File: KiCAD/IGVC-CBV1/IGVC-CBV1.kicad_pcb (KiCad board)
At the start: 2 copper layers, 9.8 x 4.5 mm, 42 parts, among them IC1 STM32F407ZGT6, IC2 SPX3819M5-L-3-3_TR, IC3 AT45DB081E-SSHN-B, J1 STLINKV2 PINS (2.54mm Pitch), J2 Motor Driver Pins (2.54mm Pit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, J3 12401948E412A, J4 Conn_01x02, SW1 SW_SPDT, Y1 EB2532YA12-25.000M_TR

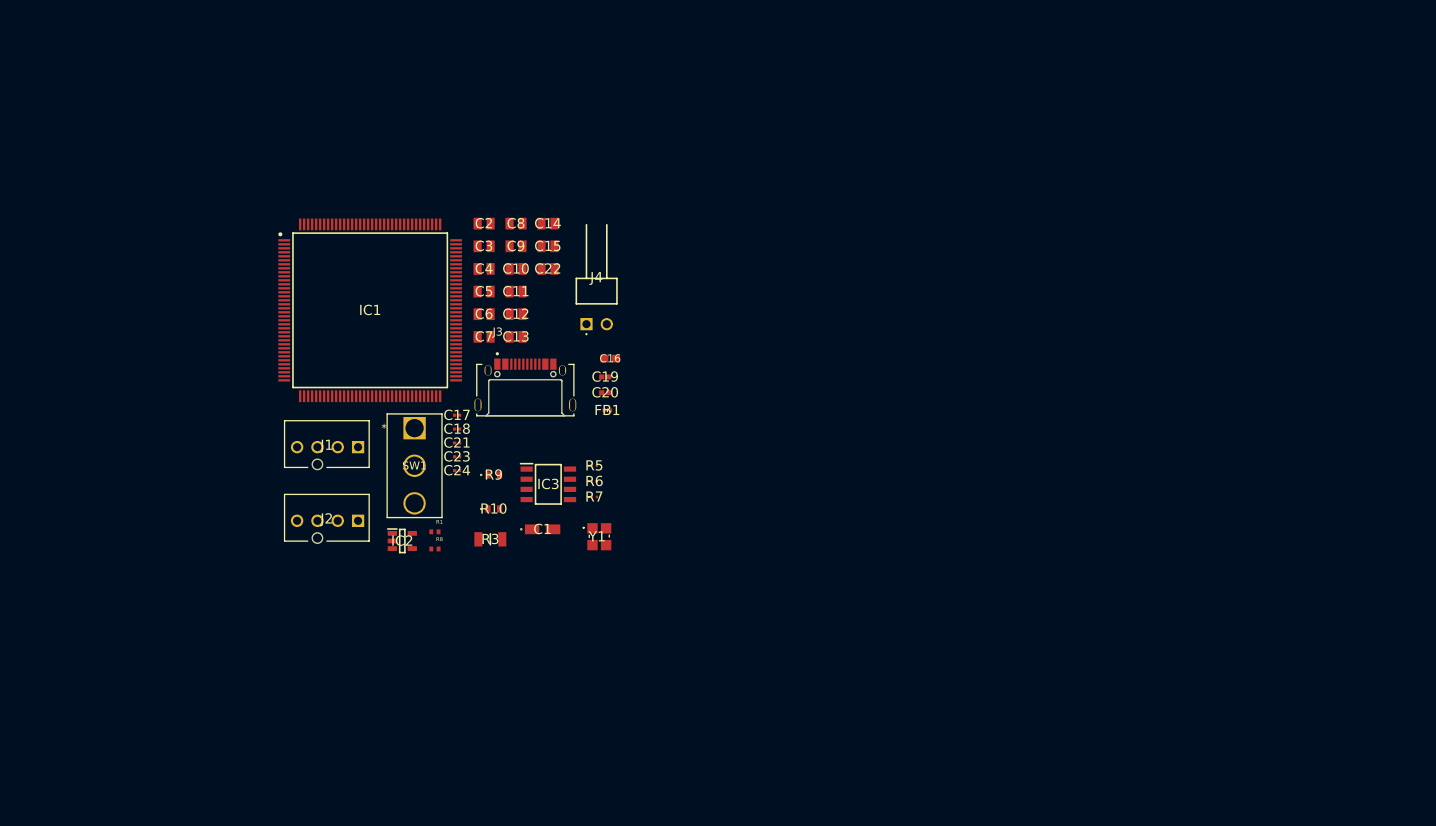
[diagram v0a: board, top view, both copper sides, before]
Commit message: placed some things where they need to go
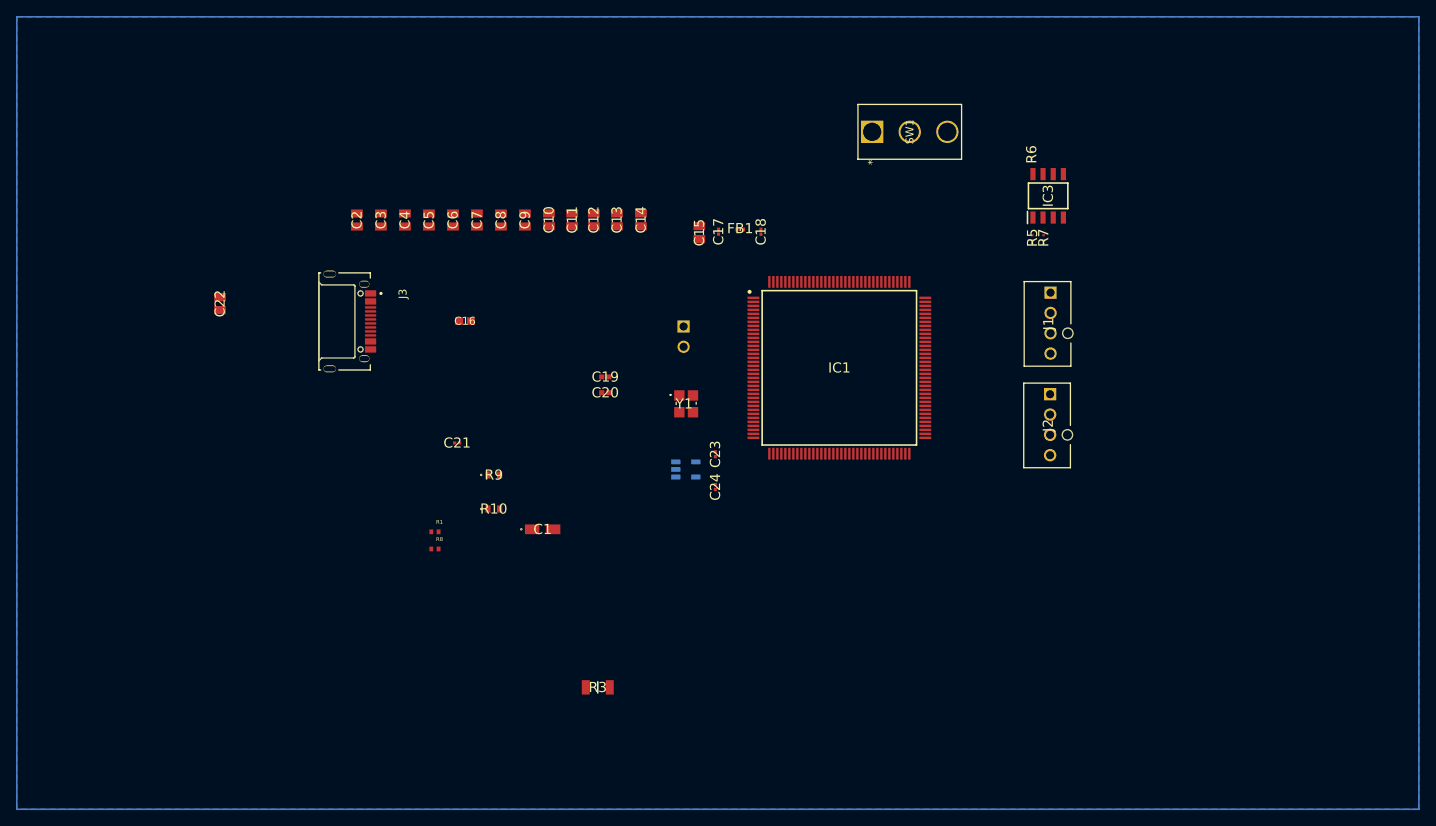
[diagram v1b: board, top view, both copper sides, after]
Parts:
- IC2, J4: moved to B.Cu
- moved J1 88.7 mm to (223.2, 80.2), turned to 90 degrees
- moved J2 87.9 mm to (223.1, 92.9), turned to 90 degrees
- moved IC3 72.1 mm to (222.9, 68.1), turned to 90 degrees
- moved R6 68.2 mm to (220.8, 62.9), turned to 90 degrees
- moved SW1 68.1 mm to (200.9, 60.1), turned to 90 degrees
- moved R7 64.8 mm to (222.3, 73.3), turned to 90 degrees
- moved R5 61.7 mm to (220.9, 73.3), turned to 90 degrees
- moved IC1 59.1 mm to (196.8, 89.6)
- moved C18 45.3 mm to (187.0, 72.6), turned to -90 degrees
- moved C22 41.2 mm to (119.4, 81.6), turned to -90 degrees
- moved C17 39.9 mm to (181.7, 72.6), turned to -90 degrees
- moved IC2 36.5 mm to (177.6, 102.3)
- moved C24 32.3 mm to (181.3, 104.5), turned to -90 degrees
- moved C23 32.3 mm to (181.3, 100.4), turned to -90 degrees
- moved FB1 28.1 mm to (184.4, 72.3)
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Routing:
- added copper zone on B.Cu, net (none)
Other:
- board size 9.8 x 4.5 mm -> 4.5 x 9.8 mm

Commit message: finished layout
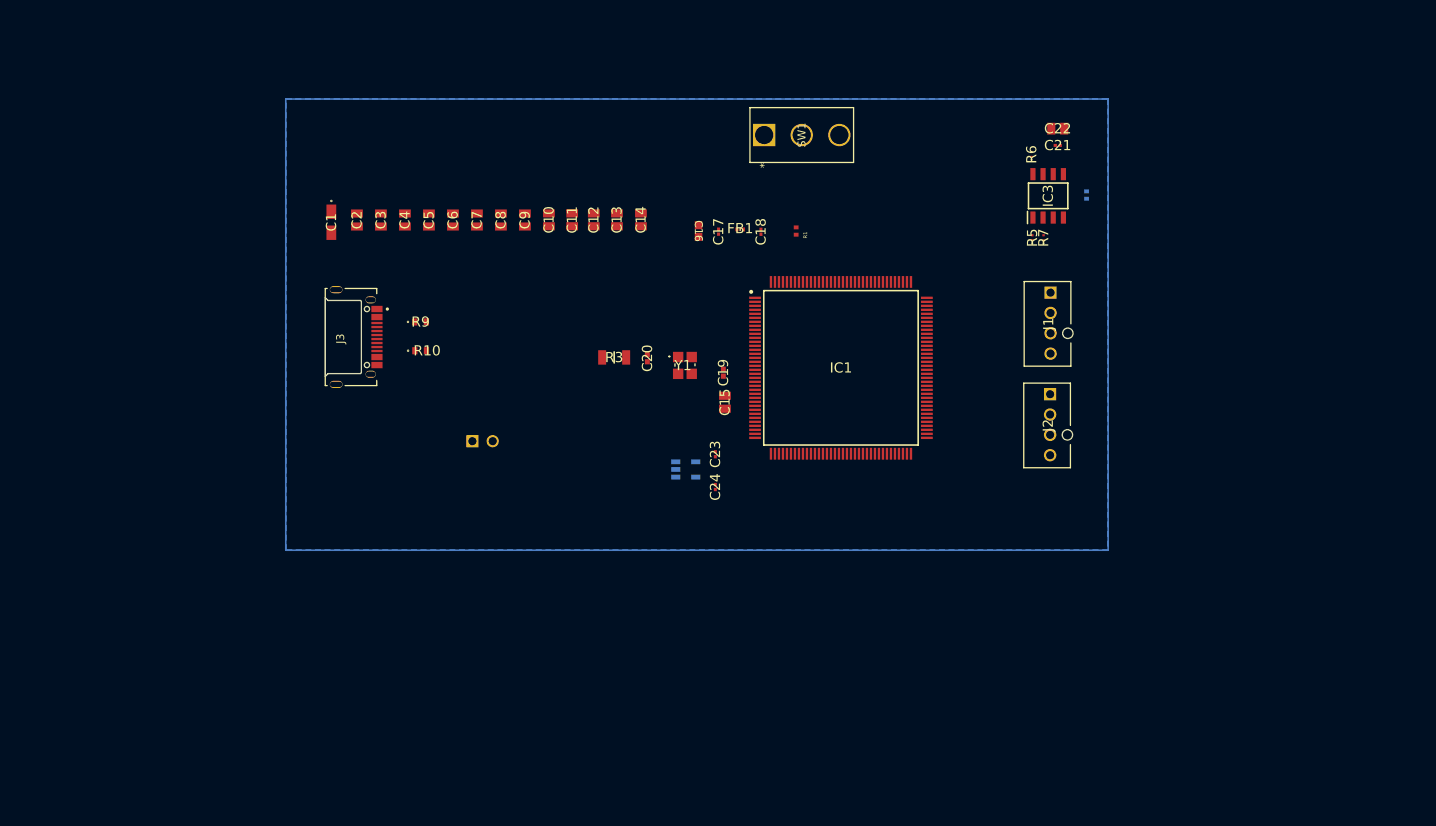
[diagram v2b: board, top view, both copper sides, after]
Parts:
- R8: moved to B.Cu
- moved C22 107.0 mm to (224.1, 59.7), turned to 180 degrees
- moved R8 92.7 mm to (227.7, 68.0), turned to 90 degrees
- moved C21 83.8 mm to (224.1, 61.8), turned to 180 degrees
- moved R1 58.8 mm to (191.4, 72.5), turned to -90 degrees
- moved C1 46.6 mm to (133.3, 71.4), turned to -90 degrees
- moved R3 41.3 mm to (168.7, 88.3), turned to 180 degrees
- moved C16 31.3 mm to (179.2, 72.5), turned to -90 degrees
- moved J4 30.0 mm to (150.9, 98.8), turned to 0 degrees
- moved R10 21.8 mm to (144.5, 87.5)
- moved C15 21.4 mm to (182.5, 93.9)
- moved R9 21.2 mm to (144.4, 83.9)
- moved C19 14.8 mm to (182.3, 90.2), turned to -90 degrees
- moved SW1 13.5 mm to (187.4, 60.5)
- moved C20 6.80 mm to (172.8, 88.4), turned to -90 degrees
- moved Y1 4.80 mm to (177.5, 89.3)
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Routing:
- added copper zone on B.Cu, net GND
- removed copper zone on B.Cu, net (none)
